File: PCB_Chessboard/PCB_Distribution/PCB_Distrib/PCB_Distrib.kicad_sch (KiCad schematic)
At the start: 12 parts, among them J1 Raspberry_Pi_4

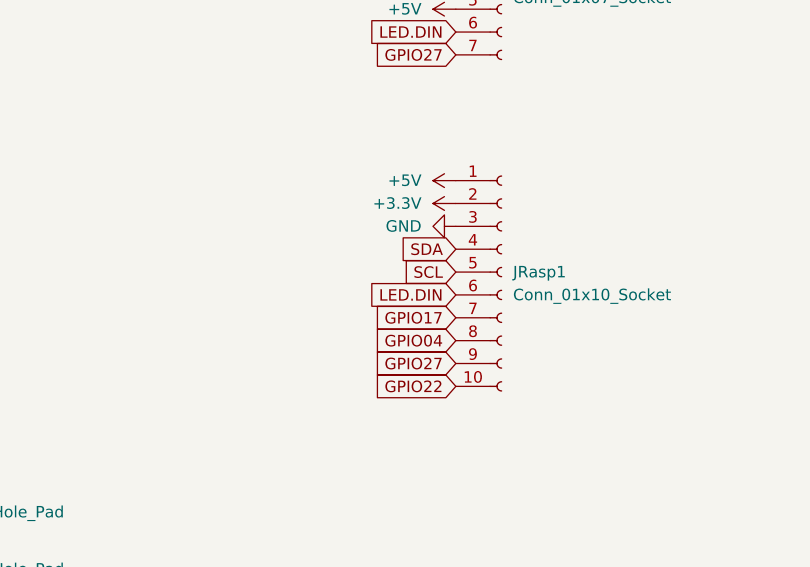
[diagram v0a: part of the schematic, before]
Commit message: update pcb
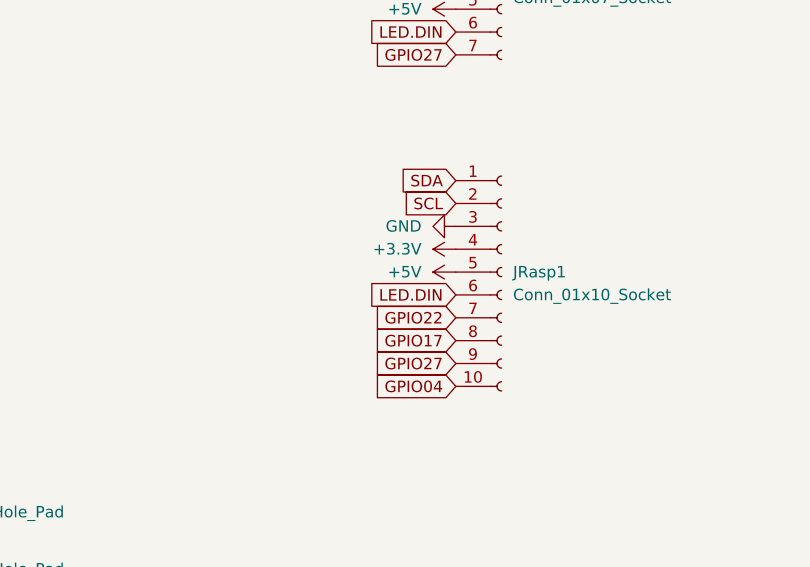
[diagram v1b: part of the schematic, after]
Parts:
- JP1, JP2, JP3, JP4: footprint Connector_JST:JST_VH_B7PS-VH_1x07_P3.96mm_Horizontal -> Connector_JST:JST_XH_B7B-XH-A_1x07_P2.50mm_Vertical
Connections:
- net +3.3V: now also JRasp1.4 (Pin_4); no longer JRasp1.2 (Pin_2)
- net +5V: now also JRasp1.5 (Pin_5); no longer JRasp1.1 (Pin_1)
- net GPIO04: now also JRasp1.10 (Pin_10); no longer JRasp1.8 (Pin_8)
- net GPIO17: now also JRasp1.8 (Pin_8); no longer JRasp1.7 (Pin_7)
- net GPIO22: now also JRasp1.7 (Pin_7); no longer JRasp1.10 (Pin_10)
- net SCL: now also JRasp1.2 (Pin_2); no longer JRasp1.5 (Pin_5)
- net SDA: now also JRasp1.1 (Pin_1); no longer JRasp1.4 (Pin_4)
